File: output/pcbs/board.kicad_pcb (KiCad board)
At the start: 2 copper layers, 160.9 x 128.6 mm, 73 parts

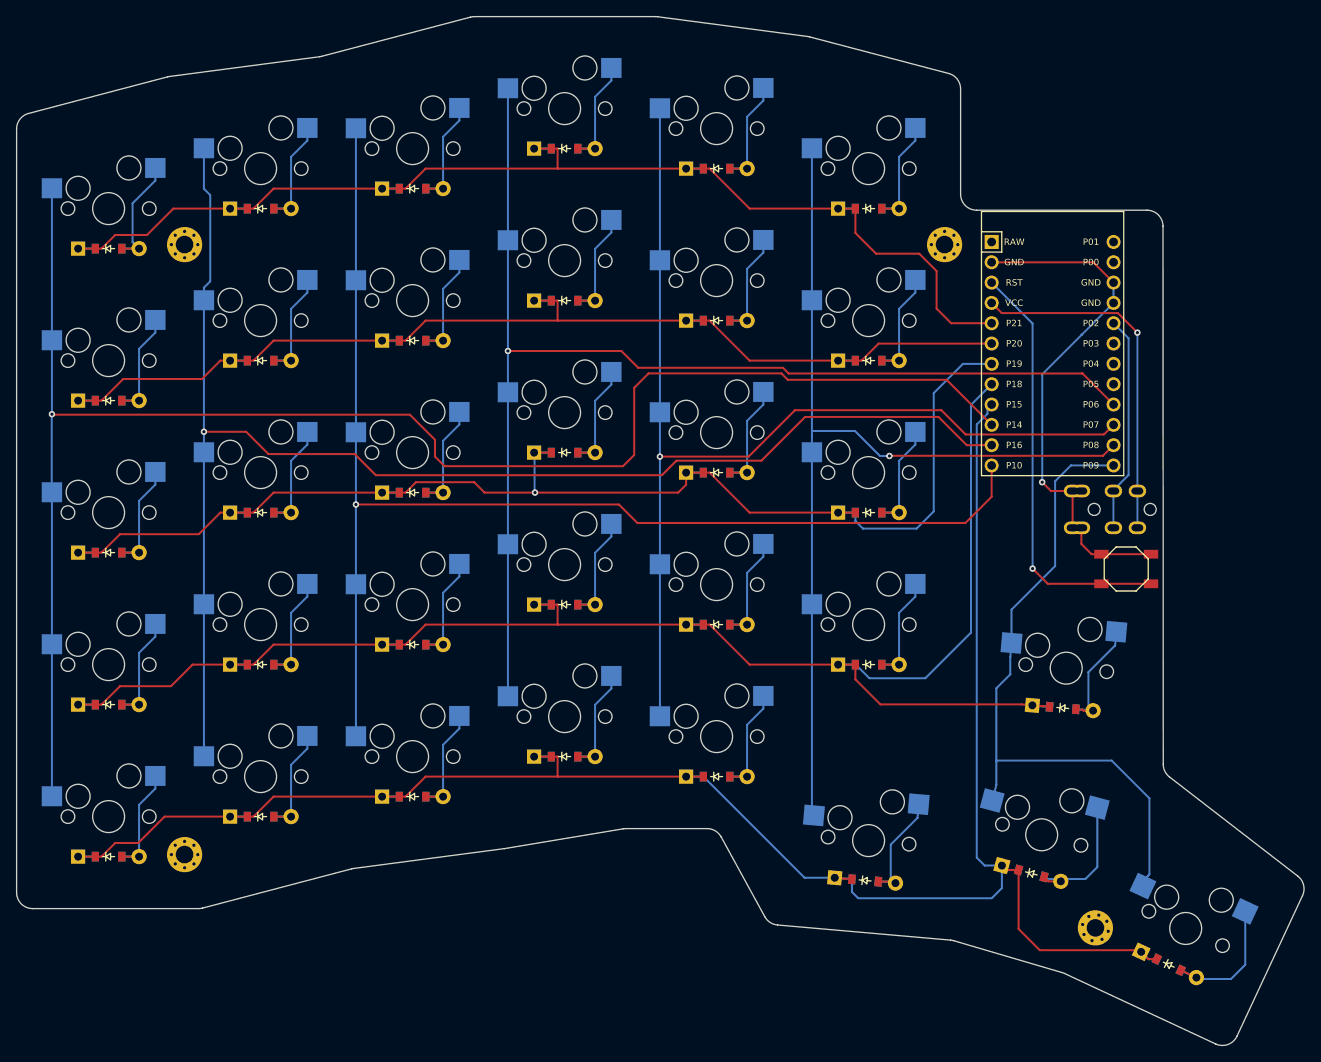
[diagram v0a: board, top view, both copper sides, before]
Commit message: Update board.kicad_pcb
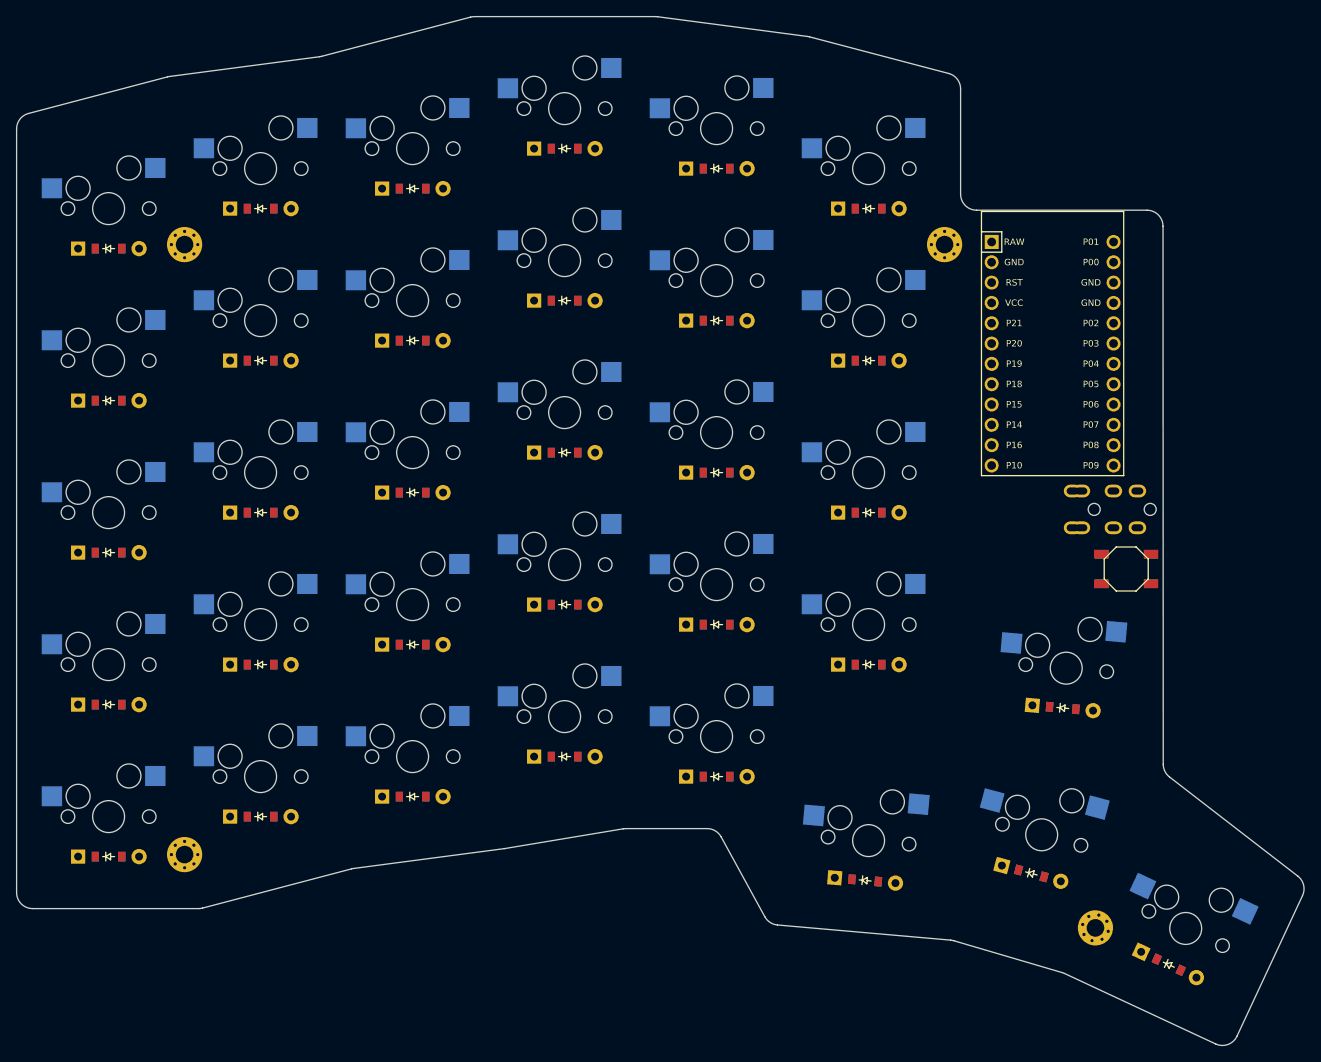
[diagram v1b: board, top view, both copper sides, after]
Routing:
- net P15: track 243.3 -> 0.00 mm
- net P14: track 209.8 -> 0.00 mm, vias 1 -> 0
- net P18: track 201.1 -> 0.00 mm
- net P16: track 181.8 -> 0.00 mm, vias 1 -> 0
- net P10: track 161.7 -> 0.00 mm, vias 1 -> 0
- net P19: track 161.1 -> 0.00 mm, vias 1 -> 0
- net P6: track 154.5 -> 0.00 mm, vias 1 -> 0
- net P21: track 149.3 -> 0.00 mm
- net P20: track 139.7 -> 0.00 mm
- net P7: track 136.9 -> 0.00 mm, vias 1 -> 0
- net P8: track 123.1 -> 0.00 mm, vias 1 -> 0
- net P9: track 83.4 -> 0.00 mm
- net GND: track 67.4 -> 0.00 mm, vias 1 -> 0
- net RST: track 53.5 -> 0.00 mm, vias 1 -> 0
- net VCC: track 44.2 -> 0.00 mm, vias 1 -> 0
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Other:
- net class Default added: clearance 0.2, trace_width 0.25, via_dia 0.8, via_drill 0.4

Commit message: Revert "Update board.kicad_pcb"
This reverts commit 021e51d17f41f71567862e83884dfb1eced45b6b.
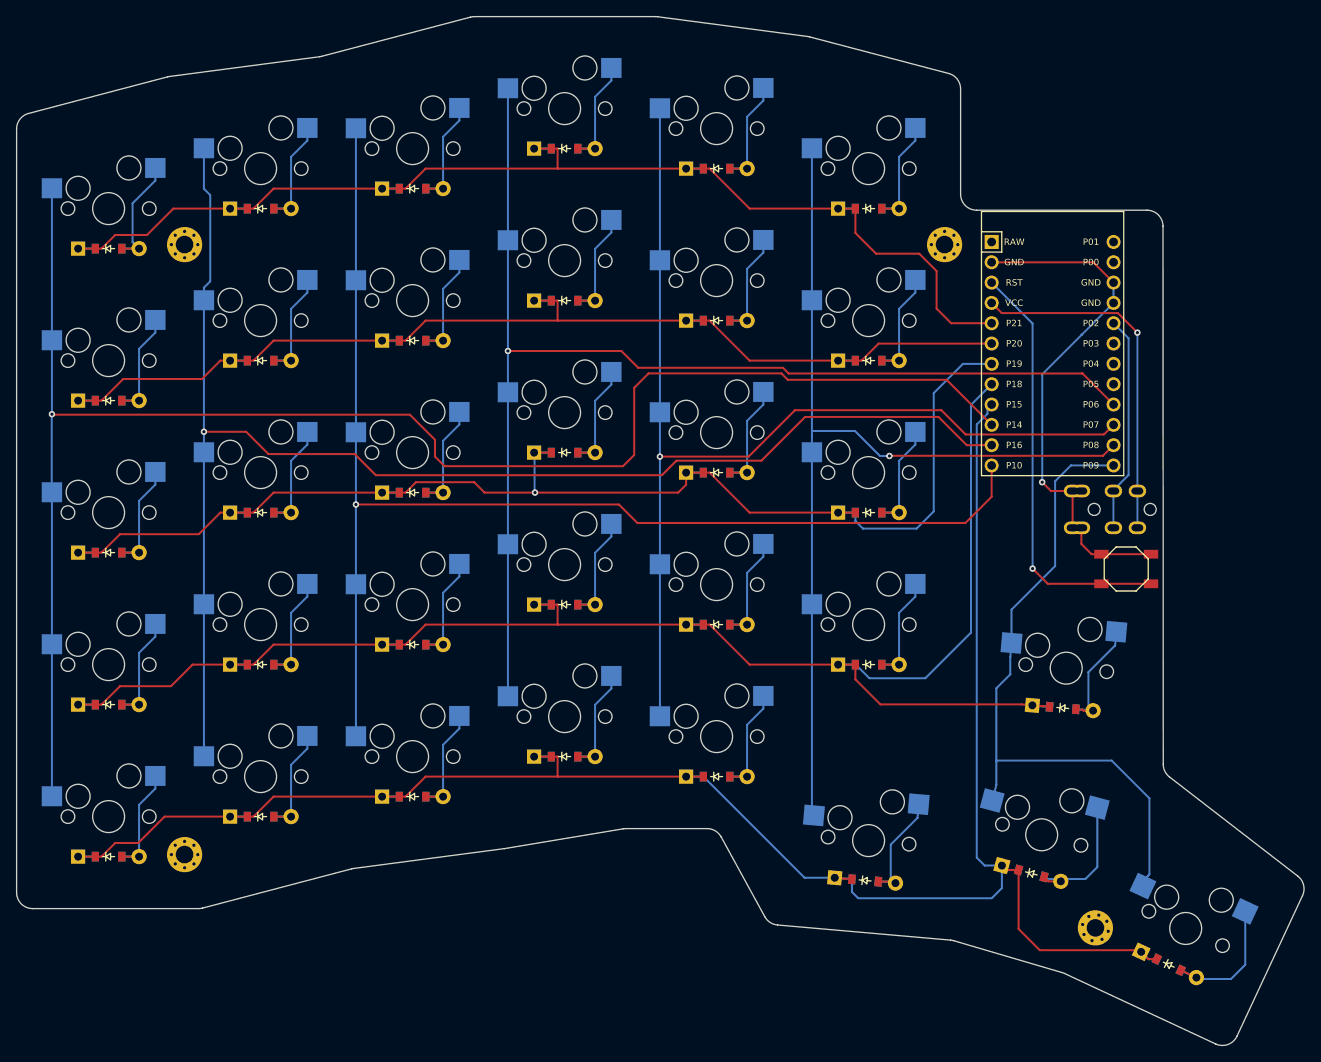
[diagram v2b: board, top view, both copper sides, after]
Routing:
- net P15: track 0.00 -> 243.3 mm
- net P14: track 0.00 -> 209.8 mm, vias 0 -> 1
- net P18: track 0.00 -> 201.1 mm
- net P16: track 0.00 -> 181.8 mm, vias 0 -> 1
- net P10: track 0.00 -> 161.7 mm, vias 0 -> 1
- net P19: track 0.00 -> 161.1 mm, vias 0 -> 1
- net P6: track 0.00 -> 154.5 mm, vias 0 -> 1
- net P21: track 0.00 -> 149.3 mm
- net P20: track 0.00 -> 139.7 mm
- net P7: track 0.00 -> 136.9 mm, vias 0 -> 1
- net P8: track 0.00 -> 123.1 mm, vias 0 -> 1
- net P9: track 0.00 -> 83.4 mm
- net GND: track 0.00 -> 67.4 mm, vias 0 -> 1
- net RST: track 0.00 -> 53.5 mm, vias 0 -> 1
- net VCC: track 0.00 -> 44.2 mm, vias 0 -> 1
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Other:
- net class Default removed
